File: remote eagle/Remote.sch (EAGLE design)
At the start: 13 parts, among them Y1 8MHz

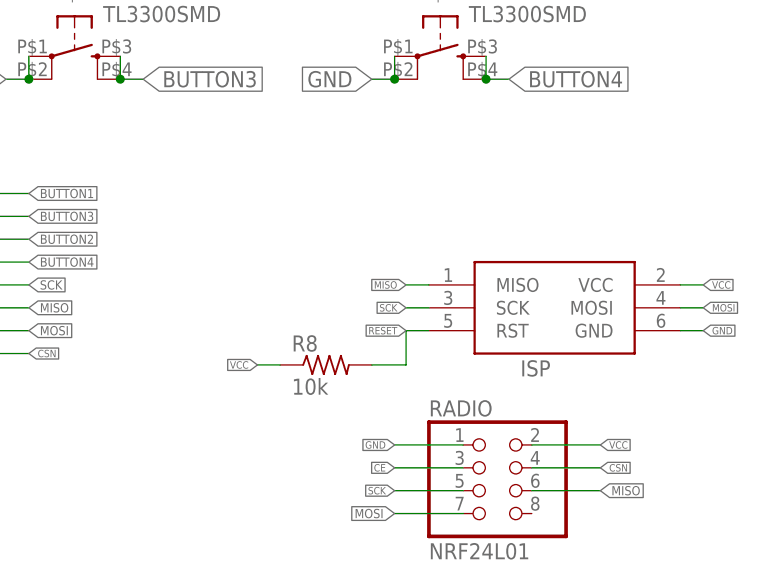
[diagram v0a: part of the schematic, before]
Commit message: Rev. 5, includes new isp touch.
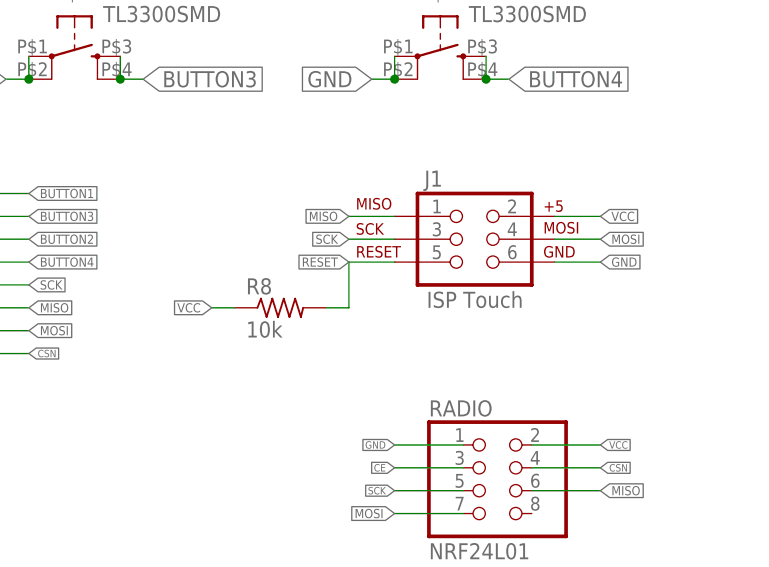
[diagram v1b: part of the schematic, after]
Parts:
- removed ISP: AVRISP-6, adafruit:AVRISP-6
- added J1: ISP Touch, remote:ISPTOUCH_HEADER
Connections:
- net GND: now also J1.6; no longer ISP.GND
- net MISO: now also J1.1; no longer ISP.MISO
- net MOSI: now also J1.4; no longer ISP.MOSI
- net RESET: now also J1.5; no longer ISP.RST
- net SCK: now also J1.3; no longer ISP.SCK
- net VCC: now also J1.2; no longer ISP.VCC
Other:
- moved on the sheet: R8
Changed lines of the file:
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@@
 <part name="ATTINY84" library="Atmel_By_element14_Batch_1" deviceset="ATTINY84-20SSU" device="" value=""/>
 <part name="C1" library="adafruit" deviceset="C-US" device="C0805" value=".1uf"/>
-<part name="ISP" library="adafruit" deviceset="AVRISP" device="-6"/>
 <part name="RADIO" library="pinhead" deviceset="PINHD-2X4" device="" value="NRF24L01"/>
 <part name="R8" library="adafruit" deviceset="R-US_" device="R0805" value="10k"/>
@@
 <part name="U$4" library="remote" deviceset="TL3300" device="SMD"/>
 <part name="U$1" library="remote" deviceset="TL3300" device="SMD"/>
+<part name="J1" library="remote" deviceset="ISPTOUCH" device="_HEADER" value="ISP Touch"/>
 </parts>
 <sheets>
@@
 <instance part="ATTINY84" gate="A" x="76.2" y="22.86"/>
 <instance part="C1" gate="G$1" x="43.18" y="20.32"/>
-<instance part="ISP" gate="G$1" x="156.21" y="15.24"/>
 <instance part="RADIO" gate="A" x="149.86" y="-5.08"/>
-<instance part="R8" gate="G$1" x="132.08" y="8.89"/>
+<instance part="R8" gate="G$1" x="127" y="15.24"/>
 <instance part="Y1" gate="G$1" x="25.4" y="-5.08" smashed="yes" rot="R90">
 <attribute name="NAME" x="26.67" y="0" size="1.778" layer="95" rot="R180"/>
@@
 <instance part="U$4" gate="G$1" x="144.78" y="45.72" rot="R270"/>
 <instance part="U$1" gate="G$1" x="22.86" y="45.72" rot="R270"/>
+<instance part="J1" gate="G$1" x="147.32" y="22.86"/>
 </instances>
 <busses>
@@
 </segment>
 <segment>
-<pinref part="ISP" gate="G$1" pin="GND"/>
-<wire x1="171.45" y1="12.7" x2="173.99" y2="12.7" width="0.1524" layer="91"/>
-<label x="173.99" y="12.7" size="0.8128" layer="95" xref="yes"/>
-</segment>
-<segment>
 <pinref part="RADIO" gate="A" pin="1"/>
 <wire x1="147.32" y1="0" x2="139.7" y2="0" width="0.1524" layer="91"/>
@@
 <pinref part="C6" gate="G$1" pin="1"/>
 </segment>
+<segment>
+<pinref part="J1" gate="G$1" pin="6"/>
+<wire x1="157.48" y1="20.32" x2="162.56" y2="20.32" width="0.1524" layer="91"/>
+<label x="162.56" y="20.32" size="1.016" layer="95" xref="yes"/>
+</segment>
 </net>
 <net name="MISO" class="0">
-<segment>
-<pinref part="ISP" gate="G$1" pin="MISO"/>
-<wire x1="143.51" y1="17.78" x2="140.97" y2="17.78" width="0.1524" layer="91"/>
-<label x="140.97" y="17.78" size="0.8128" layer="95" rot="R180" xref="yes"/>
-</segment>
 <segment>
 <pinref part="RADIO" gate="A" pin="6"/>
@@
 <label x="99.06" y="15.24" size="1.016" layer="95" xref="yes"/>
 </segment>
+<segment>
+<pinref part="J1" gate="G$1" pin="1"/>
+<wire x1="139.7" y1="25.4" x2="134.62" y2="25.4" width="0.1524" layer="91"/>
+<label x="134.62" y="25.4" size="1.016" layer="95" rot="R180" xref="yes"/>
+</segment>
 </net>
 <net name="MOSI" class="0">
-<segment>
-<pinref part="ISP" gate="G$1" pin="MOSI"/>
-<wire x1="171.45" y1="15.24" x2="173.99" y2="15.24" width="0.1524" layer="91"/>
-<label x="173.99" y="15.24" size="0.8128" layer="95" xref="yes"/>
-</segment>
 <segment>
 <pinref part="RADIO" gate="A" pin="7"/>
@@
 <label x="99.06" y="12.7" size="1.016" layer="95" xref="yes"/>
 </segment>
+<segment>
+<pinref part="J1" gate="G$1" pin="4"/>
+<wire x1="157.48" y1="22.86" x2="162.56" y2="22.86" width="0.1524" layer="91"/>
+<label x="162.56" y="22.86" size="1.016" layer="95" xref="yes"/>
+</segment>
 </net>
 <net name="SCK" class="0">
@@
 </segment>
 <segment>
-<pinref part="ISP" gate="G$1" pin="SCK"/>
-<wire x1="143.51" y1="15.24" x2="140.97" y2="15.24" width="0.1524" layer="91"/>
-<label x="140.97" y="15.24" size="0.8128" layer="95" rot="R180" xref="yes"/>
-</segment>
-<segment>
 <label x="139.7" y="-5.08" size="0.8128" layer="95" rot="R180" xref="yes"/>
 <pinref part="RADIO" gate="A" pin="5"/>
 <wire x1="139.7" y1="-5.08" x2="147.32" y2="-5.08" width="0.1524" layer="91"/>
+</segment>
+<segment>
+<pinref part="J1" gate="G$1" pin="3"/>
+<wire x1="139.7" y1="22.86" x2="134.62" y2="22.86" width="0.1524" layer="91"/>
+<label x="134.62" y="22.86" size="1.016" layer="95" rot="R180" xref="yes"/>
 </segment>
 </net>
@@
 </segment>
 <segment>
-<pinref part="ISP" gate="G$1" pin="VCC"/>
-<wire x1="171.45" y1="17.78" x2="173.99" y2="17.78" width="0.1524" layer="91"/>
-<label x="173.99" y="17.78" size="0.8128" layer="95" xref="yes"/>
-</segment>
-<segment>
 <pinref part="RADIO" gate="A" pin="2"/>
 <wire x1="154.94" y1="0" x2="162.56" y2="0" width="0.1524" layer="91"/>
@@
 </segment>
 <segment>
+<pinref part="J1" gate="G$1" pin="2"/>
+<wire x1="157.48" y1="25.4" x2="162.56" y2="25.4" width="0.1524" layer="91"/>
+<label x="162.56" y="25.4" size="1.016" layer="95" xref="yes"/>
+</segment>
+<segment>
 <pinref part="R8" gate="G$1" pin="1"/>
-<wire x1="127" y1="8.89" x2="124.46" y2="8.89" width="0.1524" layer="91"/>
-<label x="124.46" y="8.89" size="0.8128" layer="95" rot="R180" xref="yes"/>
+<wire x1="121.92" y1="15.24" x2="119.38" y2="15.24" width="0.1524" layer="91"/>
+<label x="119.38" y="15.24" size="1.016" layer="95" rot="R180" xref="yes"/>
 </segment>
 </net>
 <net name="RESET" class="0">
-<segment>
-<pinref part="ISP" gate="G$1" pin="RST"/>
-<wire x1="143.51" y1="12.7" x2="140.97" y2="12.7" width="0.1524" layer="91"/>
-<label x="140.97" y="12.7" size="0.8128" layer="95" rot="R180" xref="yes"/>
-<pinref part="R8" gate="G$1" pin="2"/>
-<wire x1="137.16" y1="8.89" x2="140.97" y2="8.89" width="0.1524" layer="91"/>
-<wire x1="140.97" y1="8.89" x2="140.97" y2="12.7" width="0.1524" layer="91"/>
-</segment>
 <segment>
 <pinref part="ATTINY84" gate="A" pin="PB3"/>
@@
 <wire x1="58.42" y1="15.24" x2="55.88" y2="15.24" width="0.1524" layer="91"/>
 </segment>
-</net>
+<segment>
+<pinref part="J1" gate="G$1" pin="5"/>
+<wire x1="139.7" y1="20.32" x2="134.62" y2="20.32" width="0.1524" layer="91"/>
+<label x="134.62" y="20.32" size="1.016" layer="95" rot="R180" xref="yes"/>
+<wire x1="134.62" y1="20.32" x2="134.62" y2="15.24" width="0.1524" layer="91"/>
+<pinref part="R8" gate="G$1" pin="2"/>
+<wire x1="134.62" y1="15.24" x2="132.08" y2="15.24" width="0.1524" layer="91"/>
+</segment>
+</net>
